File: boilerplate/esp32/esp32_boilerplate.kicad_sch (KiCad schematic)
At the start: 15 parts, among them SW1 TS-1187A-B-A-B, SW2 TS-1187A-B-A-B, U1 CH340C_C7464026, U2 AMS1117-3.3, U3 ESP32-WROOM-32E(8MB)

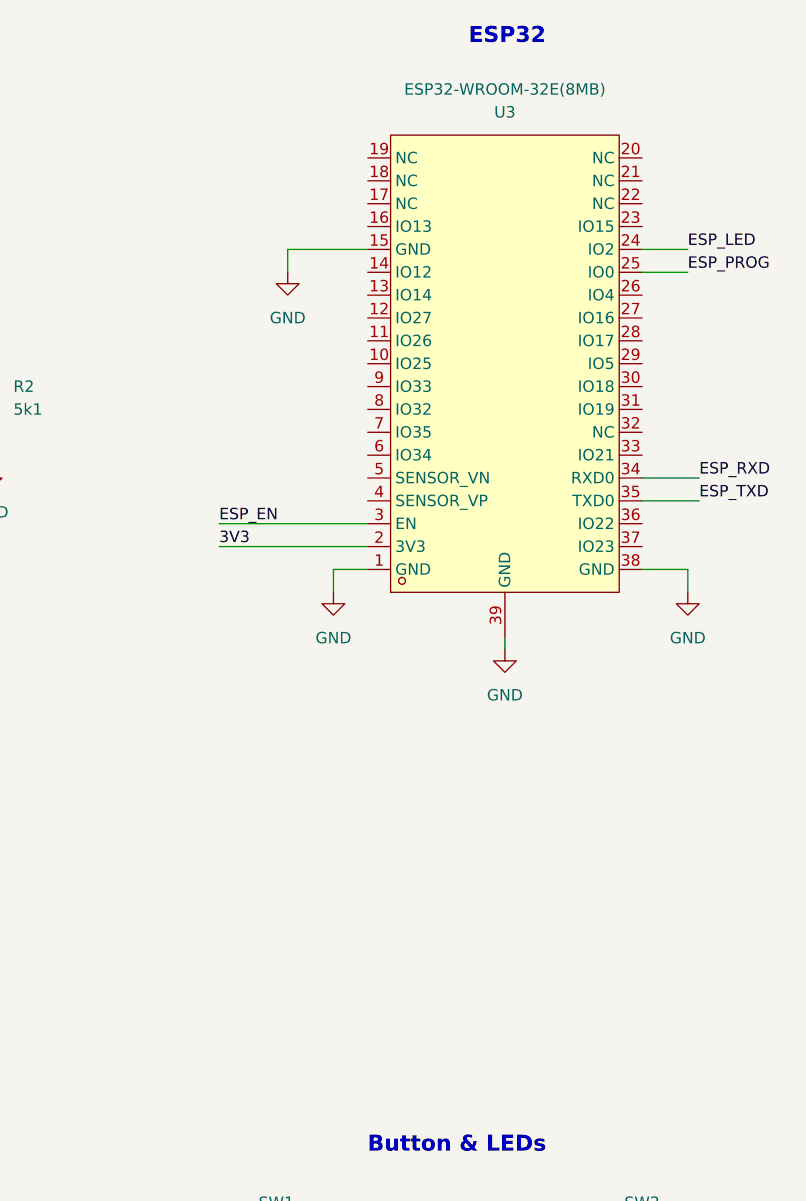
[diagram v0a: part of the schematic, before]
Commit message: Minors
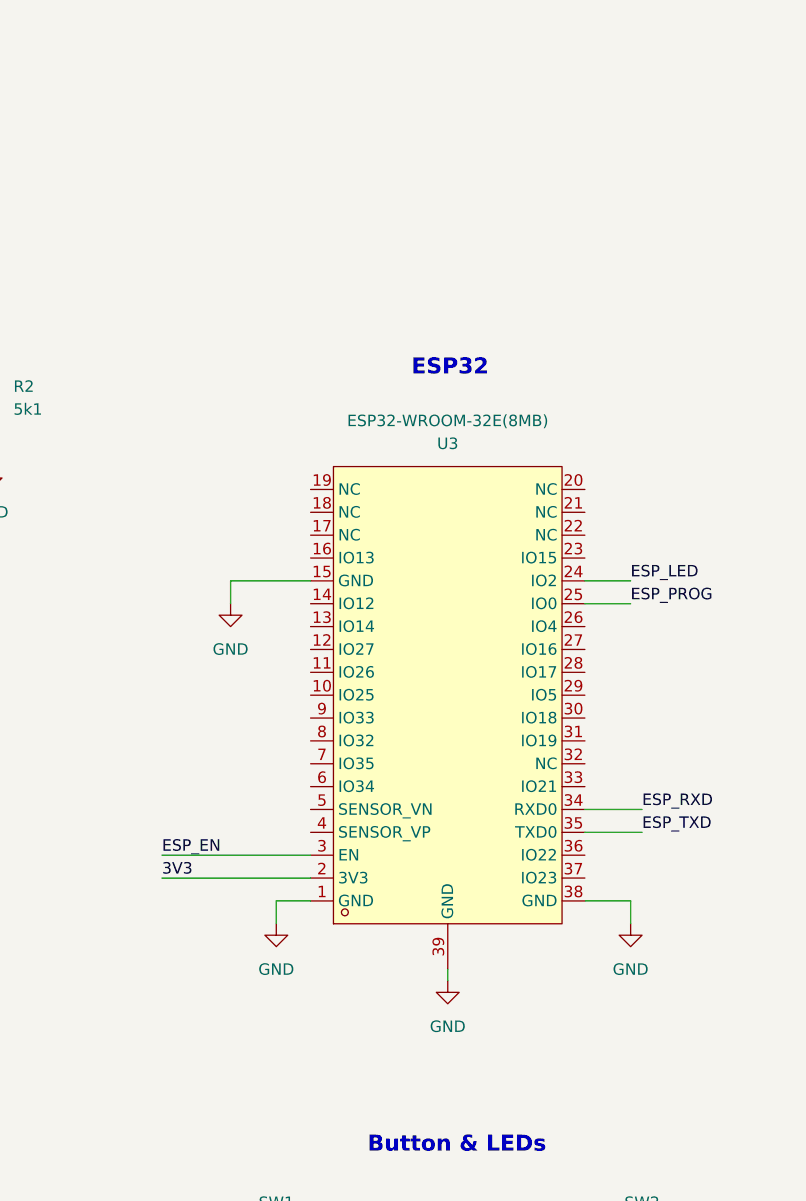
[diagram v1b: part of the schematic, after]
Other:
- moved on the sheet: U3
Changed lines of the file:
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@@
 	(wire
 		(pts
-			(xy 120.65 77.47) (xy 124.46 77.47)
+			(xy 114.3 114.3) (xy 118.11 114.3)
 		)
 		(stroke
@@
 	(wire
 		(pts
-			(xy 107.95 72.39) (xy 124.46 72.39)
+			(xy 101.6 109.22) (xy 118.11 109.22)
 		)
 		(stroke
@@
 	(wire
 		(pts
-			(xy 160.02 77.47) (xy 154.94 77.47)
+			(xy 153.67 114.3) (xy 148.59 114.3)
 		)
 		(stroke
@@
 	(wire
 		(pts
-			(xy 160.02 80.01) (xy 160.02 77.47)
+			(xy 153.67 116.84) (xy 153.67 114.3)
 		)
 		(stroke
@@
 	(wire
 		(pts
-			(xy 160.02 41.91) (xy 154.94 41.91)
+			(xy 153.67 78.74) (xy 148.59 78.74)
 		)
 		(stroke
@@
 	(wire
 		(pts
-			(xy 120.65 80.01) (xy 120.65 77.47)
+			(xy 114.3 116.84) (xy 114.3 114.3)
 		)
 		(stroke
@@
 	(wire
 		(pts
-			(xy 161.29 69.85) (xy 154.94 69.85)
+			(xy 154.94 106.68) (xy 148.59 106.68)
 		)
 		(stroke
@@
 	(wire
 		(pts
-			(xy 115.57 44.45) (xy 115.57 41.91)
+			(xy 109.22 81.28) (xy 109.22 78.74)
 		)
 		(stroke
@@
 	(wire
 		(pts
-			(xy 107.95 74.93) (xy 124.46 74.93)
+			(xy 101.6 111.76) (xy 118.11 111.76)
 		)
 		(stroke
@@
 	(wire
 		(pts
-			(xy 139.7 86.36) (xy 139.7 85.09)
+			(xy 133.35 123.19) (xy 133.35 121.92)
 		)
 		(stroke
@@
 	(wire
 		(pts
-			(xy 160.02 44.45) (xy 154.94 44.45)
+			(xy 153.67 81.28) (xy 148.59 81.28)
 		)
 		(stroke
@@
 	(wire
 		(pts
-			(xy 115.57 41.91) (xy 124.46 41.91)
+			(xy 109.22 78.74) (xy 118.11 78.74)
 		)
 		(stroke
@@
 	(wire
 		(pts
-			(xy 161.29 67.31) (xy 154.94 67.31)
+			(xy 154.94 104.14) (xy 148.59 104.14)
 		)
 		(stroke
@@
 	(text "ESP32"
 		(exclude_from_sim no)
-		(at 139.954 18.288 0)
+		(at 133.604 55.118 0)
 		(effects
 			(font
@@
 	)
 	(label "ESP_EN"
-		(at 107.95 72.39 0)
+		(at 101.6 109.22 0)
 		(fields_autoplaced yes)
 		(effects
@@
 	)
 	(label "ESP_PROG"
-		(at 160.02 44.45 0)
+		(at 153.67 81.28 0)
 		(fields_autoplaced yes)
 		(effects
@@
 	)
 	(label "ESP_LED"
-		(at 160.02 41.91 0)
+		(at 153.67 78.74 0)
 		(fields_autoplaced yes)
 		(effects
@@
 	)
 	(label "ESP_RXD"
-		(at 161.29 67.31 0)
+		(at 154.94 104.14 0)
 		(fields_autoplaced yes)
 		(effects
@@
 	)
 	(label "3V3"
-		(at 107.95 74.93 0)
+		(at 101.6 111.76 0)
 		(fields_autoplaced yes)
 		(effects
@@
 	)
 	(label "ESP_TXD"
-		(at 161.29 69.85 0)
+		(at 154.94 106.68 0)
 		(fields_autoplaced yes)
 		(effects
@@
 	(symbol
 		(lib_id "power:GND")
-		(at 120.65 80.01 0)
+		(at 114.3 116.84 0)
 		(mirror y)
 		(unit 1)
@@
 		(fields_autoplaced yes)
 		(property "Reference" "#PWR018"
-			(at 120.65 86.36 0)
+			(at 114.3 123.19 0)
 			(effects
 				(font
@@
 		)
 		(property "Value" "GND"
-			(at 120.65 85.09 0)
+			(at 114.3 121.92 0)
 			(effects
 				(font
@@
 		)
 		(property "Footprint" ""
-			(at 120.65 80.01 0)
+			(at 114.3 116.84 0)
 			(effects
 				(font
@@
 		)
 		(property "Datasheet" ""
-			(at 120.65 80.01 0)
+			(at 114.3 116.84 0)
 			(effects
 				(font
@@
 		)
 		(property "Description" "Power symbol creates a global label with name \"GND\" , ground"
-			(at 120.65 80.01 0)
+			(at 114.3 116.84 0)
 			(effects
 				(font
@@
 	(symbol
 		(lib_id "easyeda2kicad:ESP32-WROOM-32E(8MB)")
-		(at 139.7 52.07 0)
+		(at 133.35 88.9 0)
 		(mirror x)
 		(unit 1)
@@
 		(fields_autoplaced yes)
 		(property "Reference" "U3"
-			(at 139.7 26.67 0)
+			(at 133.35 63.5 0)
 			(effects
 				(font
@@
 		)
 		(property "Value" "ESP32-WROOM-32E(8MB)"
-			(at 139.7 24.13 0)
+			(at 133.35 60.96 0)
 			(effects
 				(font
@@
 		)
 		(property "Footprint" "easyeda2kicad:WIFI-SMD_ESP32-WROOM-32E"
-			(at 139.7 24.13 0)
+			(at 133.35 60.96 0)
 			(effects
 				(font
@@
 		)
 		(property "Datasheet" "https://lcsc.com/product-detail/WIFI-Modules_Espressif-Systems-ESP32-WROOM-32E-8MB_C701342.html"
-			(at 139.7 21.59 0)
+			(at 133.35 58.42 0)
 			(effects
 				(font
@@
 		)
 		(property "Description" ""
-			(at 139.7 52.07 0)
+			(at 133.35 88.9 0)
 			(effects
 				(font
@@
 		)
 		(property "LCSC Part" "C701342"
-			(at 139.7 19.05 0)
+			(at 133.35 55.88 0)
 			(effects
 				(font
@@
 	(symbol
 		(lib_id "power:GND")
-		(at 160.02 80.01 0)
+		(at 153.67 116.84 0)
 		(mirror y)
 		(unit 1)
@@
 		(fields_autoplaced yes)
 		(property "Reference" "#PWR022"
-			(at 160.02 86.36 0)
+			(at 153.67 123.19 0)
 			(effects
 				(font
@@
 		)
 		(property "Value" "GND"
-			(at 160.02 85.09 0)
+			(at 153.67 121.92 0)
 			(effects
 				(font
@@
 		)
 		(property "Footprint" ""
-			(at 160.02 80.01 0)
+			(at 153.67 116.84 0)
 			(effects
 				(font
@@
 		)
 		(property "Datasheet" ""
-			(at 160.02 80.01 0)
+			(at 153.67 116.84 0)
 			(effects
 				(font
@@
 		)
 		(property "Description" "Power symbol creates a global label with name \"GND\" , ground"
-			(at 160.02 80.01 0)
+			(at 153.67 116.84 0)
 			(effects
 				(font
@@
 	(symbol
 		(lib_id "power:GND")
-		(at 115.57 44.45 0)
+		(at 109.22 81.28 0)
 		(mirror y)
 		(unit 1)
@@
 		(fields_autoplaced yes)
 		(property "Reference" "#PWR016"
-			(at 115.57 50.8 0)
+			(at 109.22 87.63 0)
 			(effects
 				(font
@@
 		)
 		(property "Value" "GND"
-			(at 115.57 49.53 0)
+			(at 109.22 86.36 0)
 			(effects
 				(font
@@
 		)
 		(property "Footprint" ""
-			(at 115.57 44.45 0)
+			(at 109.22 81.28 0)
 			(effects
 				(font
@@
 		)
 		(property "Datasheet" ""
-			(at 115.57 44.45 0)
+			(at 109.22 81.28 0)
 			(effects
 				(font
@@
 		)
 		(property "Description" "Power symbol creates a global label with name \"GND\" , ground"
-			(at 115.57 44.45 0)
+			(at 109.22 81.28 0)
 			(effects
 				(font
@@
 	(symbol
 		(lib_id "power:GND")
-		(at 139.7 86.36 0)
+		(at 133.35 123.19 0)
 		(mirror y)
 		(unit 1)
@@
 		(fields_autoplaced yes)
 		(property "Reference" "#PWR020"
-			(at 139.7 92.71 0)
+			(at 133.35 129.54 0)
 			(effects
 				(font
@@
 		)
 		(property "Value" "GND"
-			(at 139.7 91.44 0)
+			(at 133.35 128.27 0)
 			(effects
 				(font
@@
 		)
 		(property "Footprint" ""
-			(at 139.7 86.36 0)
+			(at 133.35 123.19 0)
 			(effects
 				(font
@@
 		)
 		(property "Datasheet" ""
-			(at 139.7 86.36 0)
+			(at 133.35 123.19 0)
 			(effects
 				(font
@@
 		)
 		(property "Description" "Power symbol creates a global label with name \"GND\" , ground"
-			(at 139.7 86.36 0)
+			(at 133.35 123.19 0)
 			(effects
 				(font
